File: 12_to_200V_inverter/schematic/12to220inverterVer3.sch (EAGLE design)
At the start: 245 parts, among them IC1 UC3842, IC10 TL494, IC2 PC817, IC3 LM358SOIC8, IC4 TL431, IC5 LM317, IC6 74HC595, IC7 74HC595, IC8 ATTINY45, IC9 TL431, J2 0, J3 0, T1 AO4407AL, T10 16N60, T11 BC847, T12 BC847, T13 BSS84, T15 BC847, T16 BSS84, T17 BC847, T18 BC847, T19 BSS84, T2 IRF830, T20 BSS84, T21 BC847, T22 BC847, T23 BSS84, T24 BC847, T3 IRF830, T4 BC847, T5 BC857, T6 BC857, T7 IRFZ24N, T8 IRFZ24N, T9 BC857, X1 BAT+, X2 LAMP1, X3 LAMP1, X4 BAT-, X5 220VAC, X6 LAMP1_SWITCH, X7 LAMP1_SWITCH, X8 MCU_PROGRAMMING

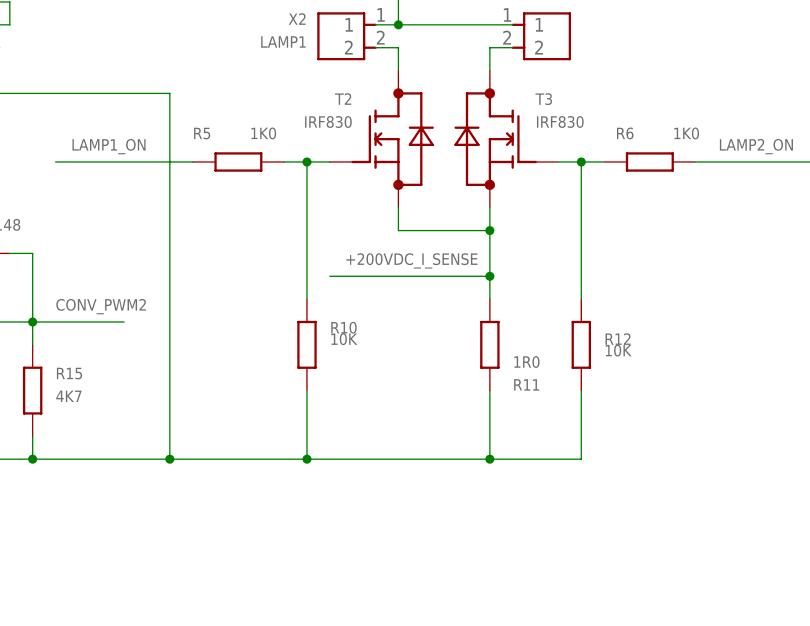
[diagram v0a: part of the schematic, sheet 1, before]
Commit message: 10 to 200V inverter. Ver3. Routing.
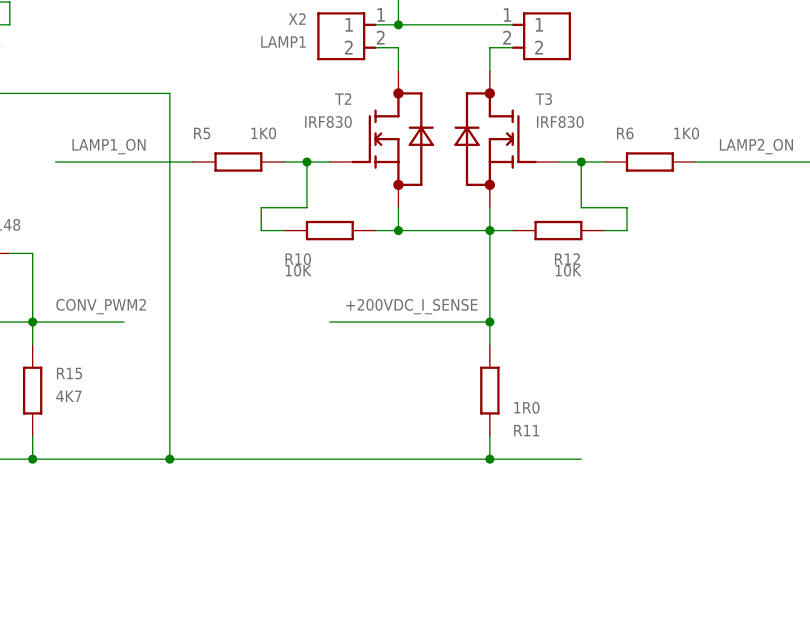
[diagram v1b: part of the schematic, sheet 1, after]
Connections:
- net +200VDC_I_SENSE: now also R10.PIN1, R12.PIN1
- net -VBAT: no longer R10.PIN1, R12.PIN1
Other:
- moved on the sheet: R10, R11, R12
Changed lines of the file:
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@@
 <attribute name="VALUE" x="132.08" y="157.48" size="1.27" layer="96" font="vector" ratio="20" rot="MR0"/>
 </instance>
-<instance part="R11" gate="R$1" x="218.44" y="124.46" smashed="yes" rot="R180">
-<attribute name="NAME" x="220.98" y="119.38" size="1.27" layer="95" font="vector" ratio="20"/>
-<attribute name="VALUE" x="220.98" y="121.92" size="1.27" layer="96" font="vector" ratio="20"/>
+<instance part="R11" gate="R$1" x="218.44" y="119.38" smashed="yes" rot="R180">
+<attribute name="NAME" x="220.98" y="114.3" size="1.27" layer="95" font="vector" ratio="20"/>
+<attribute name="VALUE" x="220.98" y="116.84" size="1.27" layer="96" font="vector" ratio="20"/>
 </instance>
 <instance part="C4" gate="C$1" x="88.9" y="157.48" smashed="yes" rot="MR0">
@@
 <attribute name="VALUE" x="191.77" y="148.59" size="1.27" layer="96" font="vector" ratio="20" rot="MR180"/>
 </instance>
-<instance part="R10" gate="R$1" x="198.12" y="124.46" smashed="yes" rot="MR180">
-<attribute name="NAME" x="200.66" y="127" size="1.27" layer="95" font="vector" ratio="20" rot="MR180"/>
-<attribute name="VALUE" x="200.66" y="125.73" size="1.27" layer="96" font="vector" ratio="20" rot="MR180"/>
+<instance part="R10" gate="R$1" x="200.66" y="137.16" smashed="yes" rot="MR90">
+<attribute name="NAME" x="195.58" y="134.62" size="1.27" layer="95" font="vector" ratio="20" rot="MR180"/>
+<attribute name="VALUE" x="195.58" y="133.35" size="1.27" layer="96" font="vector" ratio="20" rot="MR180"/>
 </instance>
 <instance part="R6" gate="R$1" x="236.22" y="144.78" smashed="yes" rot="MR270">
@@
 <attribute name="VALUE" x="238.76" y="148.59" size="1.27" layer="96" font="vector" ratio="20" rot="MR180"/>
 </instance>
-<instance part="R12" gate="R$1" x="228.6" y="124.46" smashed="yes" rot="MR180">
-<attribute name="NAME" x="231.14" y="125.73" size="1.27" layer="95" font="vector" ratio="20" rot="MR180"/>
-<attribute name="VALUE" x="231.14" y="124.46" size="1.27" layer="96" font="vector" ratio="20" rot="MR180"/>
+<instance part="R12" gate="R$1" x="226.06" y="137.16" smashed="yes" rot="MR270">
+<attribute name="NAME" x="228.6" y="133.35" size="1.27" layer="95" font="vector" ratio="20" rot="MR0"/>
+<attribute name="VALUE" x="228.6" y="132.08" size="1.27" layer="96" font="vector" ratio="20" rot="MR0"/>
 </instance>
 <instance part="T1" gate="G$1" x="71.12" y="162.56" smashed="yes" rot="MR90">
@@
 <wire x1="208.28" y1="137.16" x2="218.44" y2="137.16" width="0.1524" layer="91"/>
 <wire x1="218.44" y1="137.16" x2="218.44" y2="139.7" width="0.1524" layer="91"/>
-<wire x1="218.44" y1="129.54" x2="218.44" y2="132.08" width="0.1524" layer="91"/>
+<wire x1="218.44" y1="124.46" x2="218.44" y2="127" width="0.1524" layer="91"/>
 <junction x="218.44" y="137.16"/>
-<wire x1="218.44" y1="132.08" x2="218.44" y2="137.16" width="0.1524" layer="91"/>
-<wire x1="218.44" y1="132.08" x2="200.66" y2="132.08" width="0.1524" layer="91"/>
-<junction x="218.44" y="132.08"/>
-<label x="217.17" y="134.62" size="1.27" layer="95" font="vector" ratio="20" rot="R180"/>
+<wire x1="218.44" y1="127" x2="218.44" y2="137.16" width="0.1524" layer="91"/>
+<wire x1="218.44" y1="127" x2="200.66" y2="127" width="0.1524" layer="91"/>
+<junction x="218.44" y="127"/>
+<label x="217.17" y="129.54" size="1.27" layer="95" font="vector" ratio="20" rot="R180"/>
+<pinref part="R10" gate="R$1" pin="PIN1"/>
+<wire x1="205.74" y1="137.16" x2="208.28" y2="137.16" width="0.1524" layer="91"/>
+<pinref part="R12" gate="R$1" pin="PIN1"/>
+<wire x1="218.44" y1="137.16" x2="220.98" y2="137.16" width="0.1524" layer="91"/>
+<junction x="208.28" y="137.16"/>
 </segment>
 <segment>
@@
 <pinref part="R11" gate="R$1" pin="PIN1"/>
 <wire x1="167.64" y1="111.76" x2="182.88" y2="111.76" width="0.1524" layer="91"/>
-<wire x1="182.88" y1="111.76" x2="198.12" y2="111.76" width="0.1524" layer="91"/>
-<wire x1="198.12" y1="111.76" x2="218.44" y2="111.76" width="0.1524" layer="91"/>
-<wire x1="218.44" y1="111.76" x2="218.44" y2="119.38" width="0.1524" layer="91"/>
+<wire x1="182.88" y1="111.76" x2="218.44" y2="111.76" width="0.1524" layer="91"/>
+<wire x1="218.44" y1="111.76" x2="218.44" y2="114.3" width="0.1524" layer="91"/>
 <junction x="167.64" y="111.76"/>
-<pinref part="R10" gate="R$1" pin="PIN1"/>
-<wire x1="198.12" y1="119.38" x2="198.12" y2="111.76" width="0.1524" layer="91"/>
-<junction x="198.12" y="111.76"/>
-<pinref part="R12" gate="R$1" pin="PIN1"/>
-<wire x1="228.6" y1="119.38" x2="228.6" y2="111.76" width="0.1524" layer="91"/>
 <wire x1="228.6" y1="111.76" x2="218.44" y2="111.76" width="0.1524" layer="91"/>
 <junction x="218.44" y="111.76"/>
@@
 <wire x1="195.58" y1="144.78" x2="198.12" y2="144.78" width="0.1524" layer="91"/>
 <wire x1="198.12" y1="144.78" x2="200.66" y2="144.78" width="0.1524" layer="91"/>
-<wire x1="198.12" y1="144.78" x2="198.12" y2="129.54" width="0.1524" layer="91"/>
+<wire x1="198.12" y1="144.78" x2="198.12" y2="139.7" width="0.1524" layer="91"/>
+<wire x1="198.12" y1="139.7" x2="193.04" y2="139.7" width="0.1524" layer="91"/>
+<wire x1="193.04" y1="139.7" x2="193.04" y2="137.16" width="0.1524" layer="91"/>
+<wire x1="193.04" y1="137.16" x2="195.58" y2="137.16" width="0.1524" layer="91"/>
 <junction x="198.12" y="144.78"/>
 <pinref part="R10" gate="R$1" pin="PIN0"/>
@@
 <pinref part="R12" gate="R$1" pin="PIN0"/>
 <wire x1="228.6" y1="144.78" x2="226.06" y2="144.78" width="0.1524" layer="91"/>
-<wire x1="228.6" y1="129.54" x2="228.6" y2="144.78" width="0.1524" layer="91"/>
+<wire x1="231.14" y1="137.16" x2="233.68" y2="137.16" width="0.1524" layer="91"/>
+<wire x1="233.68" y1="137.16" x2="233.68" y2="139.7" width="0.1524" layer="91"/>
+<wire x1="233.68" y1="139.7" x2="228.6" y2="139.7" width="0.1524" layer="91"/>
+<wire x1="228.6" y1="139.7" x2="228.6" y2="144.78" width="0.1524" layer="91"/>
 <junction x="228.6" y="144.78"/>
 </segment>

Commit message: 12 to 200V inverter. Almost routed.
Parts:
- R7: device __MyCommonLib1:RSMD_1206_BIG_GAP -> __MyCommonLib1:RSMD_0805
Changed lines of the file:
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@@
 <setting verticaltext="up"/>
 </settings>
-<grid distance="0.1" unitdist="inch" unit="inch" style="lines" multiple="1" display="yes" altdistance="0.01" altunitdist="inch" altunit="inch"/>
+<grid distance="0.1" unitdist="inch" unit="inch" style="lines" multiple="1" display="no" altdistance="0.01" altunitdist="inch" altunit="inch"/>
 <layers>
-<layer number="1" name="Top" color="4" fill="1" visible="yes" active="no"/>
-<layer number="2" name="Route2" color="1" fill="3" visible="yes" active="no"/>
-<layer number="3" name="Route3" color="4" fill="3" visible="yes" active="no"/>
-<layer number="4" name="Route4" color="1" fill="4" visible="yes" active="no"/>
-<layer number="5" name="Route5" color="4" fill="4" visible="yes" active="no"/>
-<layer number="6" name="Route6" color="1" fill="8" visible="yes" active="no"/>
-<layer number="7" name="Route7" color="4" fill="8" visible="yes" active="no"/>
-<layer number="8" name="Route8" color="1" fill="2" visible="yes" active="no"/>
-<layer number="9" name="Route9" color="4" fill="2" visible="yes" active="no"/>
-<layer number="10" name="Route10" color="1" fill="7" visible="yes" active="no"/>
-<layer number="11" name="Route11" color="4" fill="7" visible="yes" active="no"/>
-<layer number="12" name="Route12" color="1" fill="5" visible="yes" active="no"/>
-<layer number="13" name="Route13" color="4" fill="5" visible="yes" active="no"/>
-<layer number="14" name="Route14" color="1" fill="6" visible="yes" active="no"/>
-<layer number="15" name="Route15" color="4" fill="6" visible="yes" active="no"/>
-<layer number="16" name="Bottom" color="1" fill="1" visible="yes" active="no"/>
-<layer number="17" name="Pads" color="2" fill="1" visible="yes" active="no"/>
-<layer number="18" name="Vias" color="2" fill="1" visible="yes" active="no"/>
-<layer number="19" name="Unrouted" color="6" fill="1" visible="yes" active="no"/>
-<layer number="20" name="Dimension" color="15" fill="1" visible="yes" active="no"/>
-<layer number="21" name="tPlace" color="7" fill="1" visible="yes" active="no"/>
-<layer number="22" name="bPlace" color="7" fill="1" visible="yes" active="no"/>
-<layer number="23" name="tOrigins" color="15" fill="1" visible="yes" active="no"/>
-<layer number="24" name="bOrigins" color="15" fill="1" visible="yes" active="no"/>
-<layer number="25" name="tNames" color="7" fill="1" visible="yes" active="no"/>
-<layer number="26" name="bNames" color="7" fill="1" visible="yes" active="no"/>
-<layer number="27" name="tValues" color="7" fill="1" visible="yes" active="no"/>
-<layer number="28" name="bValues" color="7" fill="1" visible="yes" active="no"/>
+<layer number="1" name="Top" color="4" fill="1" visible="no" active="no"/>
+<layer number="2" name="Route2" color="1" fill="3" visible="no" active="no"/>
+<layer number="3" name="Route3" color="4" fill="3" visible="no" active="no"/>
+<layer number="4" name="Route4" color="1" fill="4" visible="no" active="no"/>
+<layer number="5" name="Route5" color="4" fill="4" visible="no" active="no"/>
+<layer number="6" name="Route6" color="1" fill="8" visible="no" active="no"/>
+<layer number="7" name="Route7" color="4" fill="8" visible="no" active="no"/>
+<layer number="8" name="Route8" color="1" fill="2" visible="no" active="no"/>
+<layer number="9" name="Route9" color="4" fill="2" visible="no" active="no"/>
+<layer number="10" name="Route10" color="1" fill="7" visible="no" active="no"/>
+<layer number="11" name="Route11" color="4" fill="7" visible="no" active="no"/>
+<layer number="12" name="Route12" color="1" fill="5" visible="no" active="no"/>
+<layer number="13" name="Route13" color="4" fill="5" visible="no" active="no"/>
+<layer number="14" name="Route14" color="1" fill="6" visible="no" active="no"/>
+<layer number="15" name="Route15" color="4" fill="6" visible="no" active="no"/>
+<layer number="16" name="Bottom" color="1" fill="1" visible="no" active="no"/>
+<layer number="17" name="Pads" color="2" fill="1" visible="no" active="no"/>
+<layer number="18" name="Vias" color="2" fill="1" visible="no" active="no"/>
+<layer number="19" name="Unrouted" color="6" fill="1" visible="no" active="no"/>
+<layer number="20" name="Dimension" color="15" fill="1" visible="no" active="no"/>
+<layer number="21" name="tPlace" color="7" fill="1" visible="no" active="no"/>
+<layer number="22" name="bPlace" color="7" fill="1" visible="no" active="no"/>
+<layer number="23" name="tOrigins" color="15" fill="1" visible="no" active="no"/>
+<layer number="24" name="bOrigins" color="15" fill="1" visible="no" active="no"/>
+<layer number="25" name="tNames" color="7" fill="1" visible="no" active="no"/>
+<layer number="26" name="bNames" color="7" fill="1" visible="no" active="no"/>
+<layer number="27" name="tValues" color="7" fill="1" visible="no" active="no"/>
+<layer number="28" name="bValues" color="7" fill="1" visible="no" active="no"/>
 <layer number="29" name="tStop" color="7" fill="3" visible="no" active="no"/>
 <layer number="30" name="bStop" color="7" fill="6" visible="no" active="no"/>
@@
 <layer number="35" name="tGlue" color="7" fill="4" visible="no" active="no"/>
 <layer number="36" name="bGlue" color="7" fill="5" visible="no" active="no"/>
-<layer number="37" name="tTest" color="7" fill="1" visible="yes" active="no"/>
-<layer number="38" name="bTest" color="7" fill="1" visible="yes" active="no"/>
+<layer number="37" name="tTest" color="7" fill="1" visible="no" active="no"/>
+<layer number="38" name="bTest" color="7" fill="1" visible="no" active="no"/>
 <layer number="39" name="tKeepout" color="4" fill="11" visible="no" active="no"/>
 <layer number="40" name="bKeepout" color="1" fill="11" visible="no" active="no"/>
@@
 <layer number="44" name="Drills" color="7" fill="1" visible="no" active="no"/>
 <layer number="45" name="Holes" color="7" fill="1" visible="no" active="no"/>
-<layer number="46" name="Milling" color="3" fill="1" visible="yes" active="no"/>
-<layer number="47" name="Measures" color="7" fill="1" visible="yes" active="no"/>
-<layer number="48" name="Document" color="7" fill="1" visible="yes" active="no"/>
-<layer number="49" name="Reference" color="7" fill="1" visible="yes" active="no"/>
-<layer number="51" name="tDocu" color="7" fill="1" visible="yes" active="no"/>
-<layer number="52" name="bDocu" color="7" fill="1" visible="yes" active="no"/>
+<layer number="46" name="Milling" color="3" fill="1" visible="no" active="no"/>
+<layer number="47" name="Measures" color="7" fill="1" visible="no" active="no"/>
+<layer number="48" name="Document" color="7" fill="1" visible="no" active="no"/>
+<layer number="49" name="Reference" color="7" fill="1" visible="no" active="no"/>
+<layer number="51" name="tDocu" color="7" fill="1" visible="no" active="no"/>
+<layer number="52" name="bDocu" color="7" fill="1" visible="no" active="no"/>
 <layer number="91" name="Nets" color="2" fill="1" visible="yes" active="yes"/>
 <layer number="92" name="Busses" color="1" fill="1" visible="yes" active="yes"/>
@@
 <part name="R4" library="__MyCommonLib1" deviceset="R" device="SMD_0805" value="10K"/>
 <part name="T4" library="__MyCommonLib1" deviceset="BC847" device="SOT23_SMALL_PADS" value="BC847"/>
-<part name="R7" library="__MyCommonLib1" deviceset="R" device="SMD_1206_BIG_GAP" value="1K0"/>
+<part name="R7" library="__MyCommonLib1" deviceset="R" device="SMD_0805" value="1K0"/>
 <part name="R13" library="__MyCommonLib1" deviceset="R" device="SMD_0805" value="10K"/>
 <part name="R8" library="__MyCommonLib1" deviceset="R" device="SMD_0805" value="10K"/>

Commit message: 12 to 200V inverter. Routed.
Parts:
- D21: device __MyCommonLib1:1N4001DO-41_12.5MM -> __MyCommonLib1:1N4001DO-41_10MM
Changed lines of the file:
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@@
 <part name="GND30" library="supply1" deviceset="GND" device=""/>
 <part name="R98" library="__MyCommonLib1" deviceset="R" device="SMD_0805" value="10K"/>
-<part name="D21" library="__MyCommonLib1" deviceset="1N4001" device="DO-41_12.5MM" value="1N4001"/>
+<part name="D21" library="__MyCommonLib1" deviceset="1N4001" device="DO-41_10MM" value="1N4001"/>
 <part name="T1" library="__MyCommonLib1" deviceset="AO4407" device="(SO8)" value="AO4407AL"/>
 <part name="R1" library="__MyCommonLib1" deviceset="R" device="SMD_1206" value="1R0"/>
